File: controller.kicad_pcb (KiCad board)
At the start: 2 copper layers, 25 parts, among them J1 Conn_01x04, J2 Conn_01x08, J3 Conn_01x16, SW1 SW_Push, U1 PRTR5V0U2X, U2 AT90USB1286-AU, Y1 16MHz

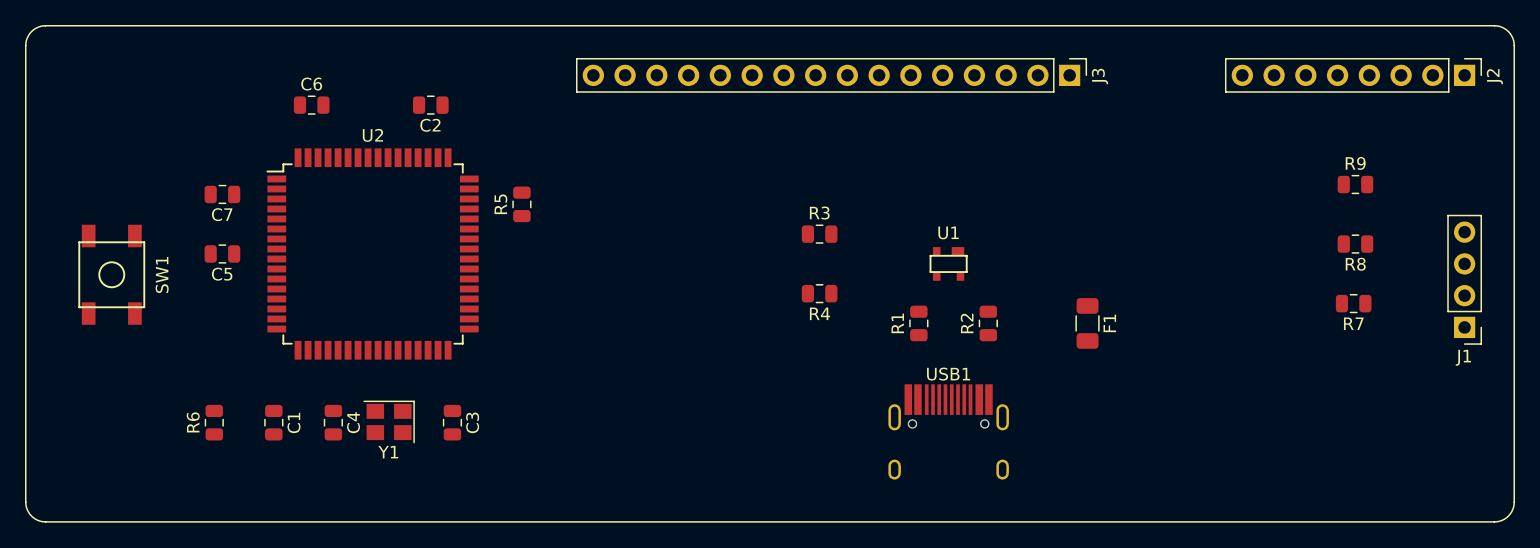
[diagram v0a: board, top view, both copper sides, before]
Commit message: completion?! finished all circuitry
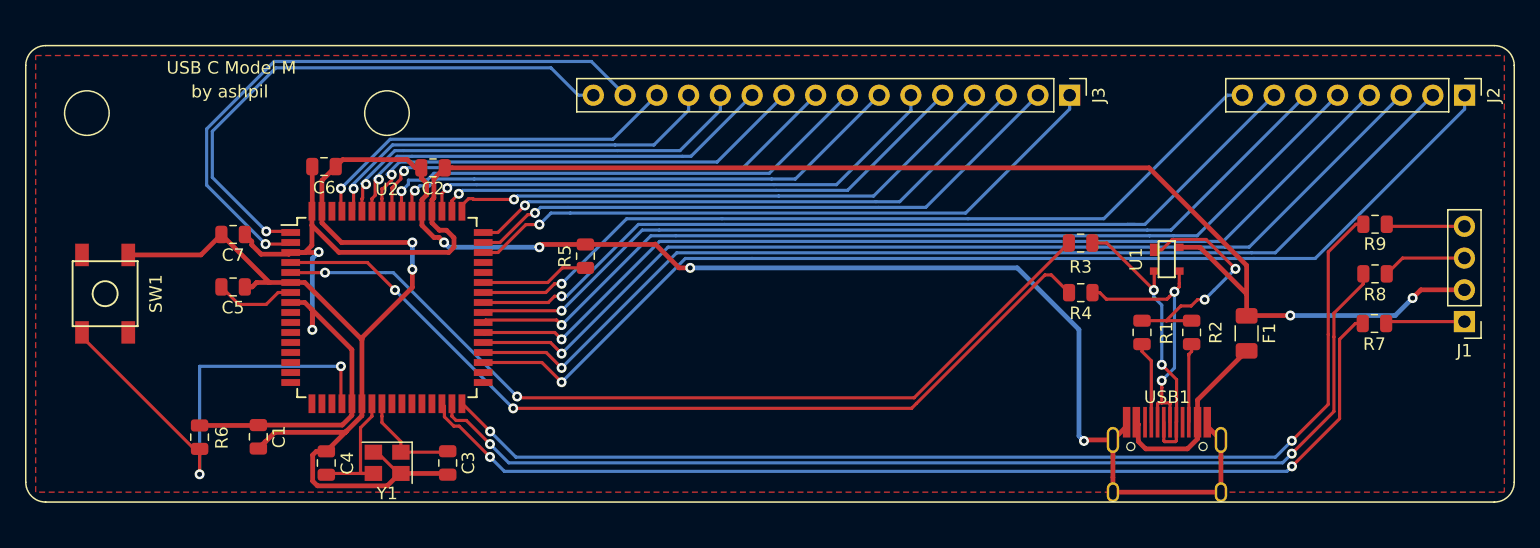
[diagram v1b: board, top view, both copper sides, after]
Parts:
- moved R4 20.9 mm to (124.1, 92.8)
- moved R3 20.9 mm to (124.1, 88.8)
- moved R1 17.9 mm to (129.0, 96.0)
- moved USB1 17.6 mm to (131.0, 111.3)
- moved U1 17.5 mm to (131.0, 90.1), turned to 270 degrees
- moved R2 16.3 mm to (132.9, 96.0)
- moved F1 12.7 mm to (137.3, 96.0)
- moved R5 6.55 mm to (84.5, 89.9)
- moved C2 5.02 mm to (72.3, 82.8)
- moved C6 5.01 mm to (63.5, 82.7)
- moved U2 4.42 mm to (68.6, 94.0)
- moved R9 3.54 mm to (147.6, 87.3)
- moved C7 3.31 mm to (56.3, 88.1)
- moved C4 3.28 mm to (63.7, 106.4)
- moved Y1 3.27 mm to (68.6, 106.4)
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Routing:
- net GND: track 0.00 -> 183.3 mm, vias 0 -> 6
- net +5V: track 0.00 -> 164.2 mm, vias 0 -> 4
- net Net-(J2-Pad1): track 0.00 -> 89.3 mm, vias 0 -> 1
- net Net-(R9-Pad1): track 0.00 -> 88.7 mm, vias 0 -> 2
- net Net-(R8-Pad2): track 0.00 -> 86.8 mm, vias 0 -> 2
- net Net-(J2-Pad2): track 0.00 -> 85.5 mm, vias 0 -> 1
- net Net-(R7-Pad2): track 0.00 -> 85.0 mm, vias 0 -> 2
- net Net-(J2-Pad3): track 0.00 -> 82.4 mm, vias 0 -> 1
- net Net-(J2-Pad4): track 0.00 -> 79.3 mm, vias 0 -> 1
- net Net-(J2-Pad5): track 0.00 -> 76.3 mm, vias 0 -> 1
- net Net-(J2-Pad6): track 0.00 -> 73.0 mm, vias 0 -> 1
- net Net-(R4-Pad2): track 0.00 -> 72.1 mm, vias 0 -> 2
- net Net-(R3-Pad1): track 0.00 -> 71.5 mm, vias 0 -> 2
- net Net-(J2-Pad7): track 0.00 -> 70.7 mm, vias 0 -> 1
- net Net-(J2-Pad8): track 0.00 -> 67.3 mm, vias 0 -> 1
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- added copper zone on F.Cu, net GND
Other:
- board text added: "USB C Model M"
- board text added: "by ashpil"
